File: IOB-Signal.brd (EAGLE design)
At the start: 20.3 x 50.8 mm, 25 parts, among them CON1 RJ45, IC1 74HS139A, Q0 MOSFET-P, Q1 MOSFET-P, Q2 MOSFET-P, Q3 MOSFET-P

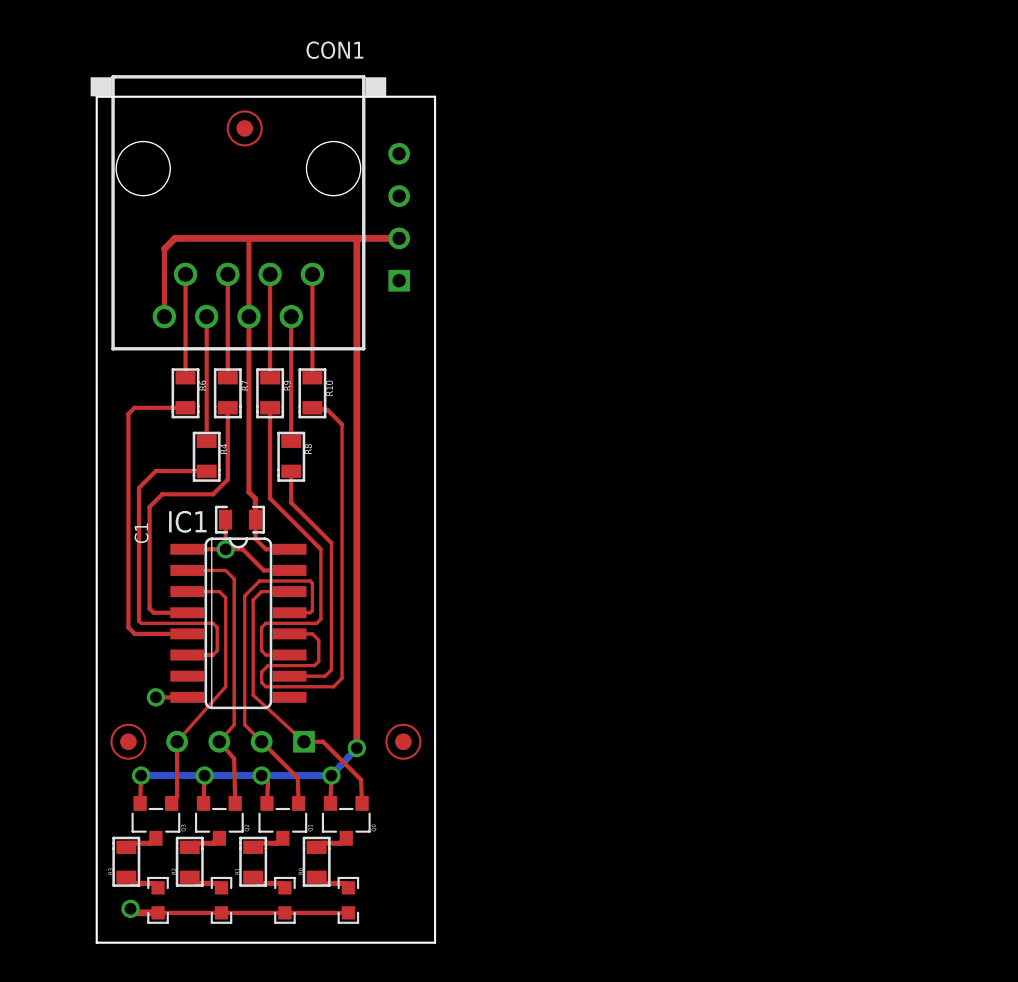
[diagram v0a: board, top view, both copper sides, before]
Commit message: new IOB format
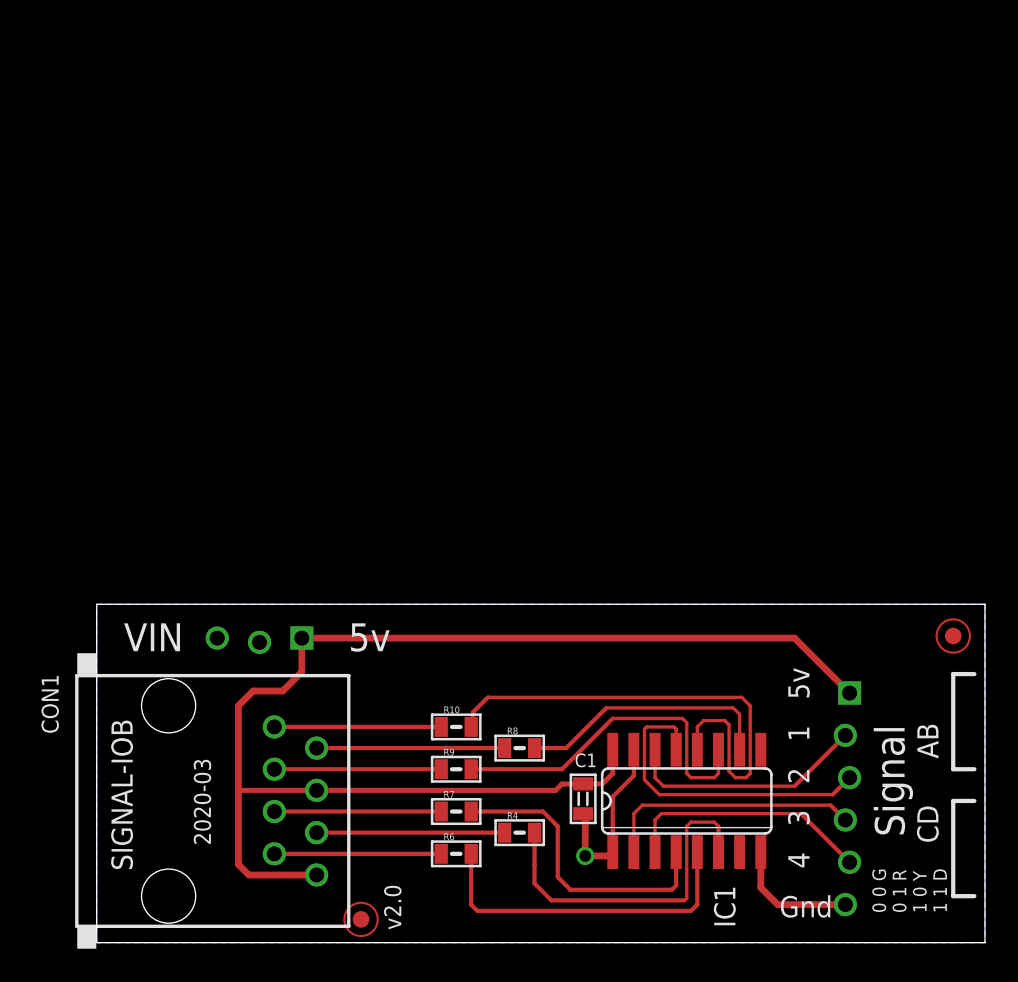
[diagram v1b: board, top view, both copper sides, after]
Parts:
- removed FID2: FIDUCIAL, SPCoast:FIDUCIAL_1MM
- removed IOB: IO4-IOBBARE, SPCoast:IO4-IOB
- removed LED0, LED1, LED2, LED3: Y, SPCoast:0603-LED
- removed Q0, Q1, Q2, Q3: MOSFET-P, SPCoast:SOT23-3
- removed R0, R1, R2, R3: 2K2, SPCoast:0805-RES
- added U$1: CONNECTOR-IO4-IOBBARE, SPCoast:IO4-IOB
- moved FID1 48.0 mm to (15.9, 1.40), turned to 0 degrees
- moved CON1 38.2 mm to (4.32, 8.51), turned to 270 degrees
- moved FID3 33.6 mm to (51.4, 18.4), turned to 0 degrees
- moved R6 32.1 mm to (21.6, 5.33), turned to 0 degrees
- moved R4 29.4 mm to (25.4, 6.60), turned to 0 degrees
- moved IC1 29.0 mm to (35.4, 8.51), turned to 0 degrees
- moved R7 28.6 mm to (21.6, 7.87), turned to 0 degrees
- moved C1 26.5 mm to (29.2, 8.64), turned to 270 degrees
- moved R9 25.2 mm to (21.6, 10.4), turned to 0 degrees
- moved R8 22.3 mm to (25.4, 11.7), turned to 0 degrees
- moved R10 21.8 mm to (21.6, 13.0), turned to 0 degrees
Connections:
- removed net N$11: Q0.3, R0.2
- removed net N$2: LED0.A, R0.1
- removed net N$3: LED1.A, R1.1
- removed net N$30: Q1.3, R1.2
- removed net N$31: Q2.3, R2.2
- removed net N$32: Q3.3, R3.2
- removed net N$4: LED2.A, R2.1
- removed net N$5: LED3.A, R3.1
- net GND: now also U$1.G@3; no longer IOB.G@1, IOB.G@2, LED0.C, LED1.C, LED2.C, LED3.C
- net P1: now also U$1.P1; no longer IOB.P1, Q0.1
- net P2: now also U$1.P2; no longer IOB.P2, Q1.1
- net P3: now also U$1.P3; no longer IOB.P3, Q2.1
- net P4: now also U$1.P4; no longer IOB.P4, Q3.1
- net VCC: now also U$1.V5, U$1.V5@1; no longer IOB.V5, Q0.2, Q1.2, Q2.2, Q3.2
- net VCCIO: now also U$1.V+; no longer IOB.V+
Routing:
- net VCC: track 90.1 -> 79.8 mm, vias 5 -> 0
- net GND: track 23.5 -> 18.7 mm, vias 3 -> 1
- net R2-LED: track 6.21 -> 10.0 mm
- net R1-LED: track 6.21 -> 10.0 mm
- net G2-LED: track 6.21 -> 10.0 mm
- net G1-LED: track 6.21 -> 10.0 mm
- net Y2-LED: track 7.48 -> 11.3 mm
- net Y1-LED: track 7.48 -> 11.3 mm
- net P1: track 18.0 -> 14.6 mm
- net N$3: track 2.17 -> 0.00 mm
- net N$5: track 2.17 -> 0.00 mm
- net N$2: track 2.17 -> 0.00 mm
- net N$4: track 2.14 -> 0.00 mm
- net N$31: track 1.98 -> 0.00 mm
- net N$32: track 1.98 -> 0.00 mm
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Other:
- board size 20.3 x 50.8 mm -> 53.3 x 20.3 mm
- board text added: "2020-03"
- board text added: "AB"
- board text added: "Blue Soldermask White Silkscreen"
- board text added: "C1"
- board text added: "CD"
- board text added: "CON1"
- board text added: "IC1"
- board text added: "R10"
- board text added: "R4"
- board text added: "R6"
- board text added: "R7"
- board text added: "R8"
- board text added: "R9"
- board text added: "SIGNAL-IOB"
- board text added: "v2.0"
- board text removed: "IO Interface"
- board text removed: "IO4-IOB"
- board text removed: "Made in the PCR, Coast Div, NMRA"
- board text removed: "Model Railroading is Fun!"
- board text removed: "v1.1"
